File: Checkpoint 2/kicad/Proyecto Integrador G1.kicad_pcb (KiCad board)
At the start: 2 copper layers, 96.5 x 81.3 mm, 54 parts, among them J1 Conn_01x02, J2 Conn_01x02, Q1 BC547, Q10 BC547, Q2 BC547, Q3 BC547, Q4 BC547, Q5 BC557, Q6 BC557, Q7 BC547, Q8 TIP42C, Q9 BC547, U1 TL431LP, U2 LM358

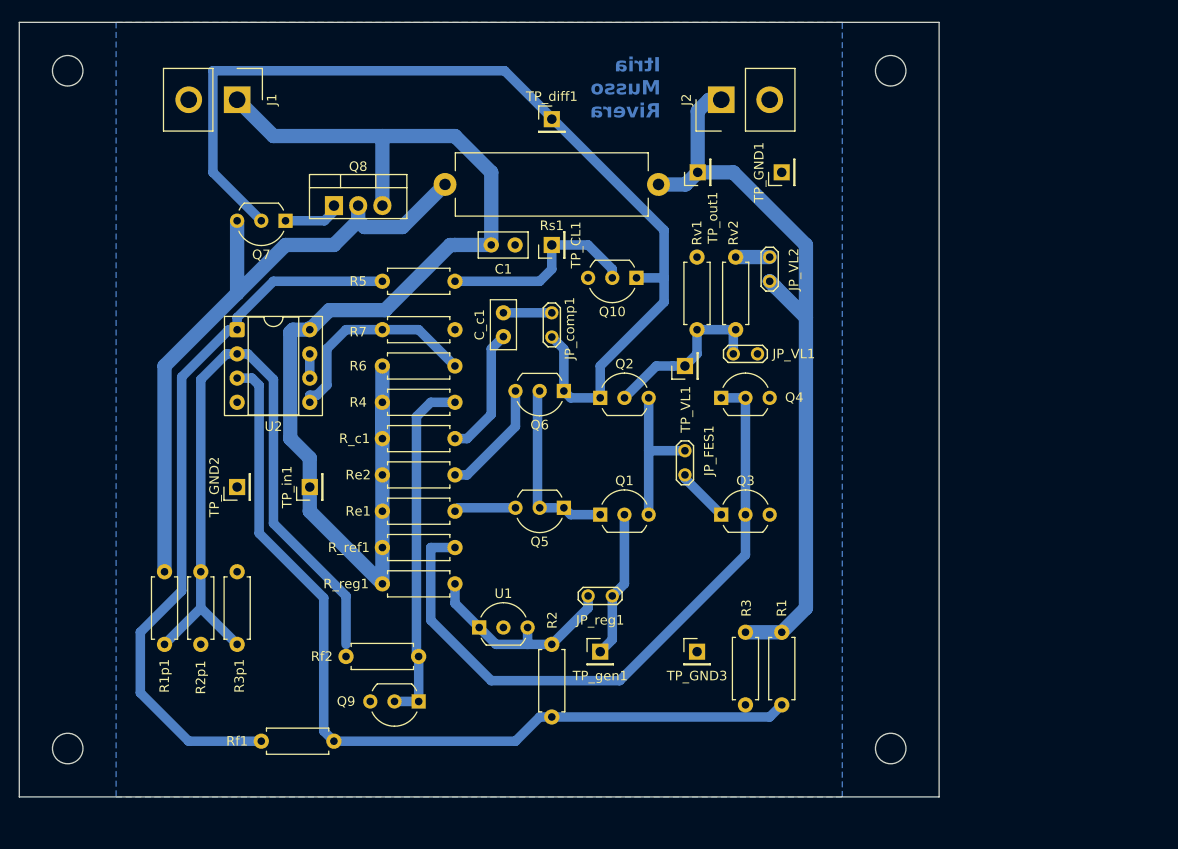
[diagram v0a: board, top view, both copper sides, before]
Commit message: rev 1.2
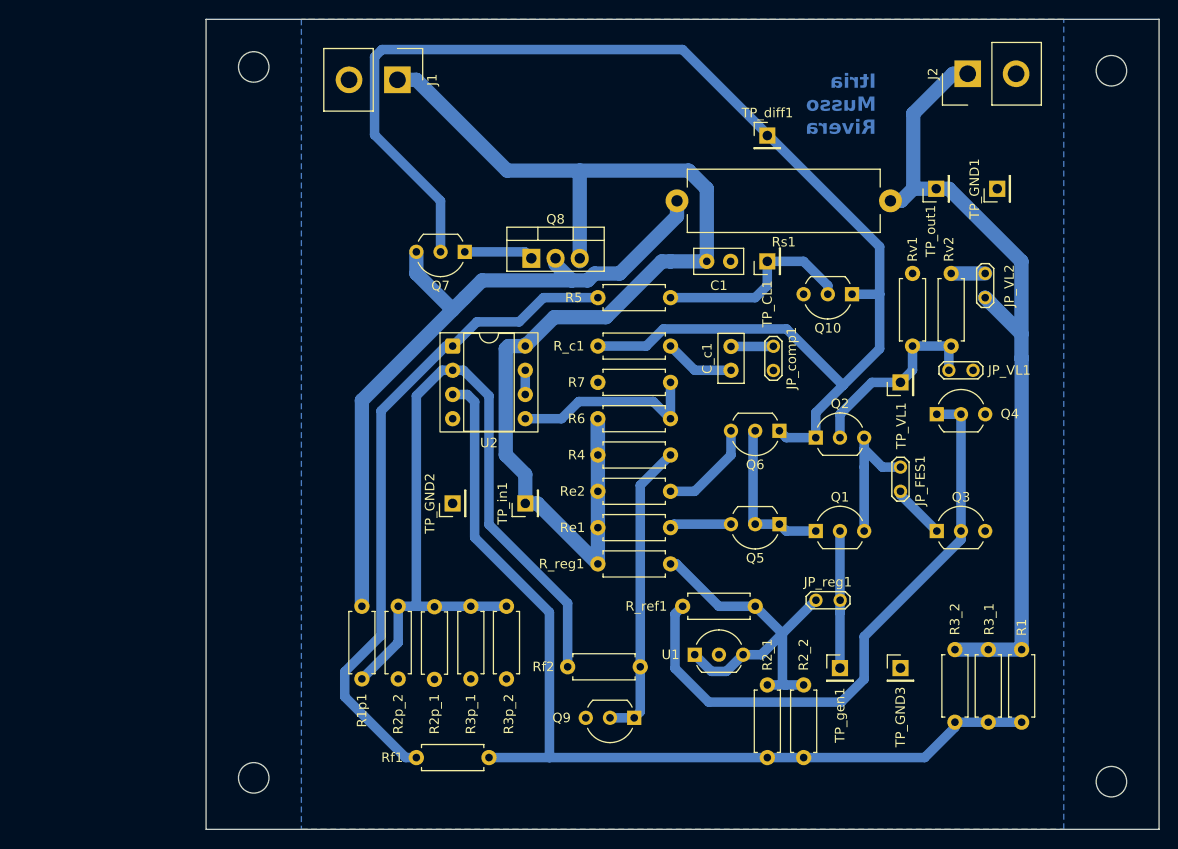
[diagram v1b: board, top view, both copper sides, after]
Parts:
- added R2_2: 1M, Resistor_THT:R_Axial_DIN0207_L6.3mm_D2.5mm_P7.62mm_Horizontal, F.Cu at (107.7, 89.8)
- added R2p_2: 1M, Resistor_THT:R_Axial_DIN0207_L6.3mm_D2.5mm_P7.62mm_Horizontal, F.Cu at (65.2, 89.2)
- added R3_2: 1M, Resistor_THT:R_Axial_DIN0207_L6.3mm_D2.5mm_P7.62mm_Horizontal, F.Cu at (123.6, 86.1)
- added R3p_2: 1M, Resistor_THT:R_Axial_DIN0207_L6.3mm_D2.5mm_P7.62mm_Horizontal, F.Cu at (76.5, 89.2)
- C1: value 100nF -> 100n
- C_c1: value 100n -> 1u
- Q8: value TIP42C -> TIP32C
- R2_1: renamed from R2; value 500k -> 1M
- R2p_1: renamed from R2p1; value 500k -> 1M
- R3_1: renamed from R3; value 500k -> 1M
- R3p_1: renamed from R3p1; value 500k -> 1M
- R_ref1: value 3k3 -> 1k
- moved R3p_1 27.0 mm to (72.8, 89.2), turned to 90 degrees
- moved J2 26.0 mm to (124.9, 25.7)
- moved R3_1 25.5 mm to (127.1, 86.1)
- moved R1 25.2 mm to (130.6, 86.1)
- moved TP_gen1 25.2 mm to (111.5, 88.1)
- moved TP_out1 25.1 mm to (121.6, 37.8)
- moved R2p_1 24.8 mm to (69.0, 89.3)
- moved R_ref1 24.7 mm to (95.0, 81.6), turned to 0 degrees
- moved R_c1 24.6 mm to (86.1, 54.3)
- moved Rs1 24.4 mm to (116.8, 39.0)
- moved C_c1 24.1 mm to (100.1, 56.8)
- moved JP_reg1 23.9 mm to (109.0, 81.0)
- moved REF** 23.4 mm to (140.0, 100.0)
- moved R6 23.3 mm to (93.7, 61.9)
- moved R4 23.3 mm to (86.1, 65.7)
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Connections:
- C_c1 pad 2: Net-(JP_comp1-B) -> Net-(JP_comp1-A)
- JP_comp1 pad 1: Vb -> Net-(JP_comp1-A)
- JP_comp1 pad 2: Net-(JP_comp1-B) -> GND
- R_c1 pad 1: Vref -> Vb
- R_ref1 pad 2: Vref -> Vreg
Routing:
- net Vb: track 105.7 -> 144.0 mm
- net Vreg: track 22.4 -> 40.6 mm
- net Net-(U2A-+): track 91.8 -> 101.0 mm
- net Net-(U2A--): track 75.6 -> 84.3 mm
- net Net-(Q3-B): track 70.3 -> 63.7 mm
- net Vout: track 80.3 -> 86.8 mm
- net Net-(R5-Pad1): track 75.7 -> 69.4 mm
- net Vfold: track 68.7 -> 75.0 mm
- net Net-(C_c1-Pad1): track 13.5 -> 7.40 mm
- net Net-(Q9-B): track 37.2 -> 31.7 mm
- net Net-(JP_comp1-B): track 5.08 -> 0.00 mm
- net Net-(JP_comp1-A): track 0.00 -> 4.45 mm
- net Net-(JP_VL1-B): track 18.8 -> 21.2 mm
- net Net-(Q1-C): track 19.0 -> 16.6 mm
- net Net-(U2B-+): track 22.6 -> 20.5 mm
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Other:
- board size 96.5 x 81.3 mm -> 100 x 85 mm
